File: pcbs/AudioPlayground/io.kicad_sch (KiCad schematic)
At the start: 24 parts, among them J1 Conn_01x07_Socket, J2 Conn_Battery, J5 Conn_01x12_Pin, J7 Conn_01x16_Pin, J9 Conn_01x07_Socket, U19 GTD3526BA-1N, U20 GTD3526BA-1N, U7 DMM-4326-T-R, U8 DMM-4326-T-R

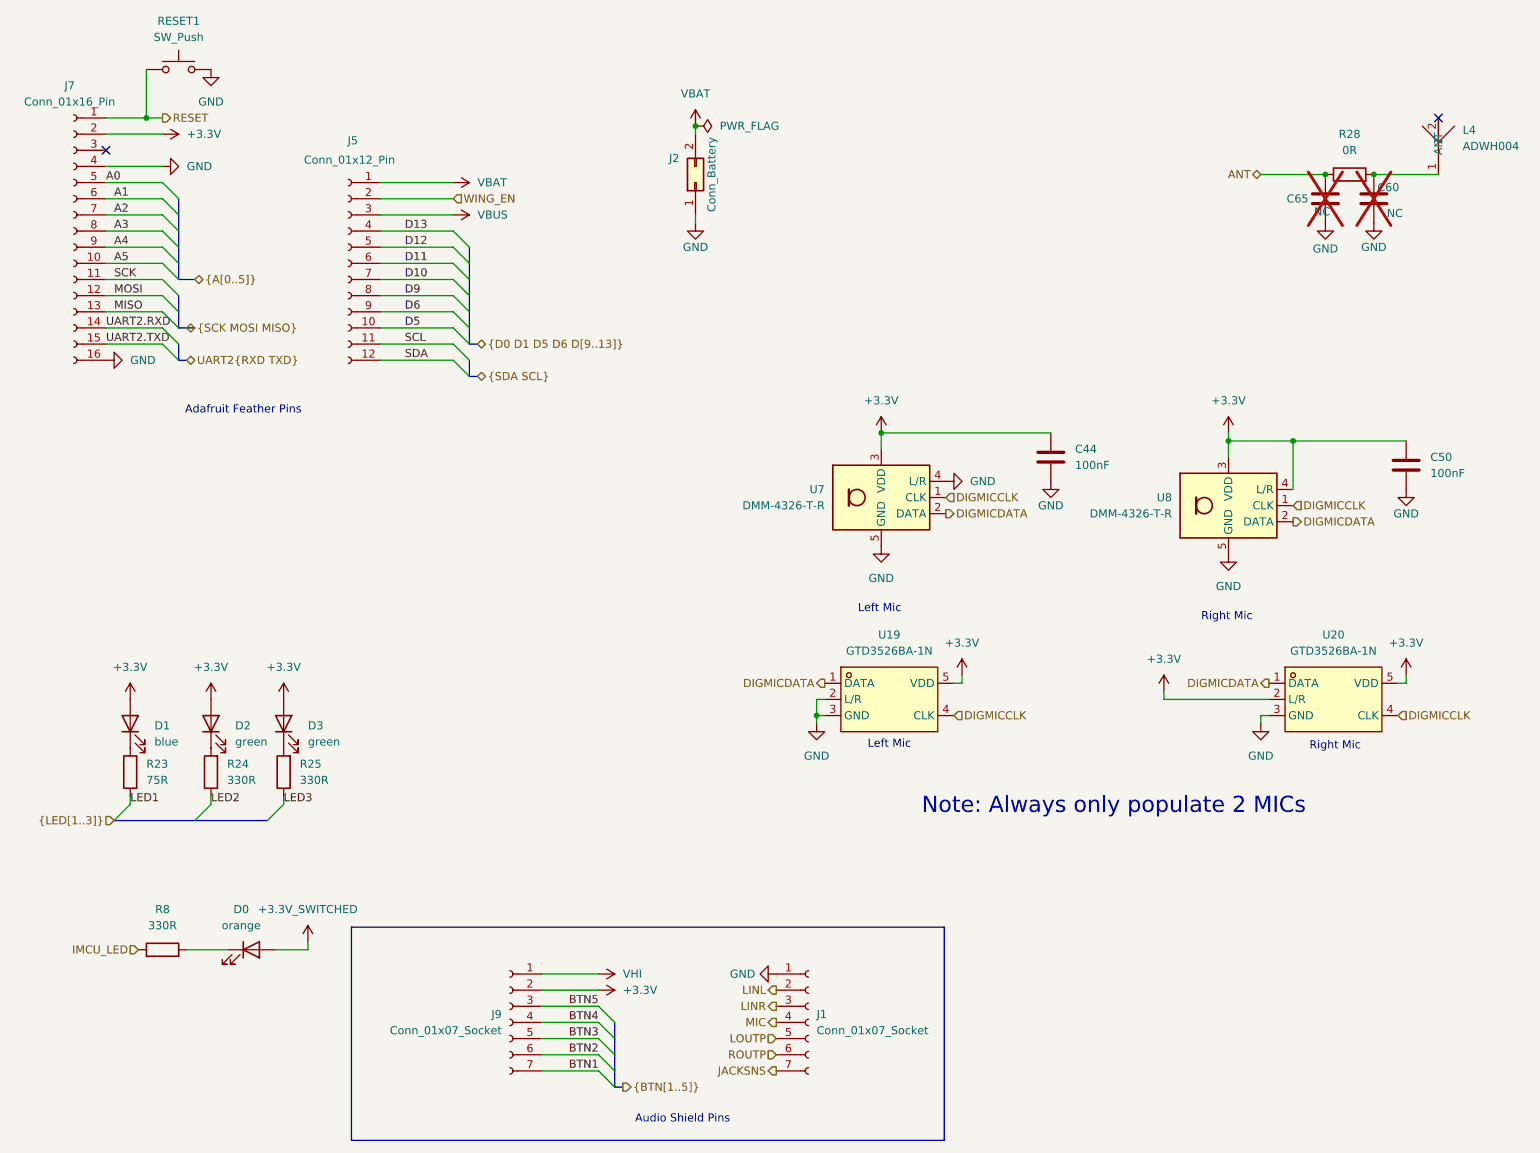
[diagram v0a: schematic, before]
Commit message: Improve Optic
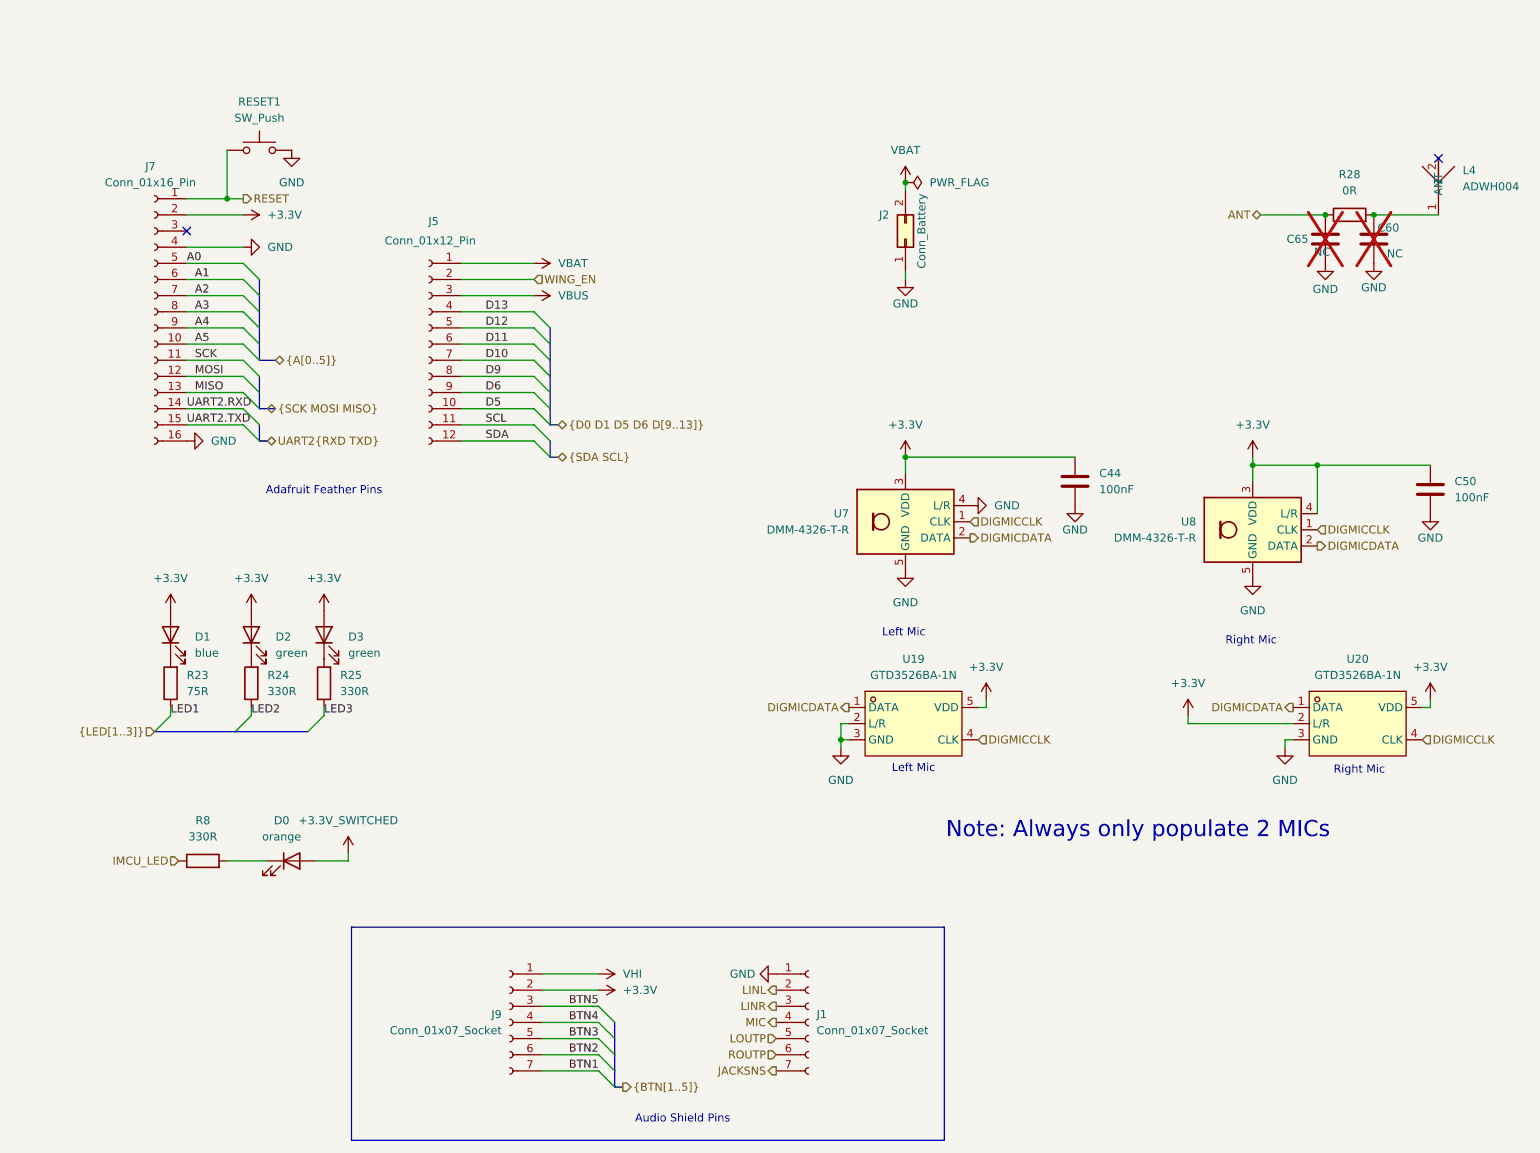
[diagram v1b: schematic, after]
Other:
- title: (none) -> LE Audio Playground
- moved on the sheet: C44, C50, C60, C65, D0, D1, D2, D3, J2, J5, J7, L4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
